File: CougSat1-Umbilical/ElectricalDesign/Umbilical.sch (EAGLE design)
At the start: 48 parts, among them J1 USB, J2 Umbilical, J3 5V input, Q1 CSD16406Q3, Q2 CSD16406Q3, U1 FT230XQ, U2 BQ24650

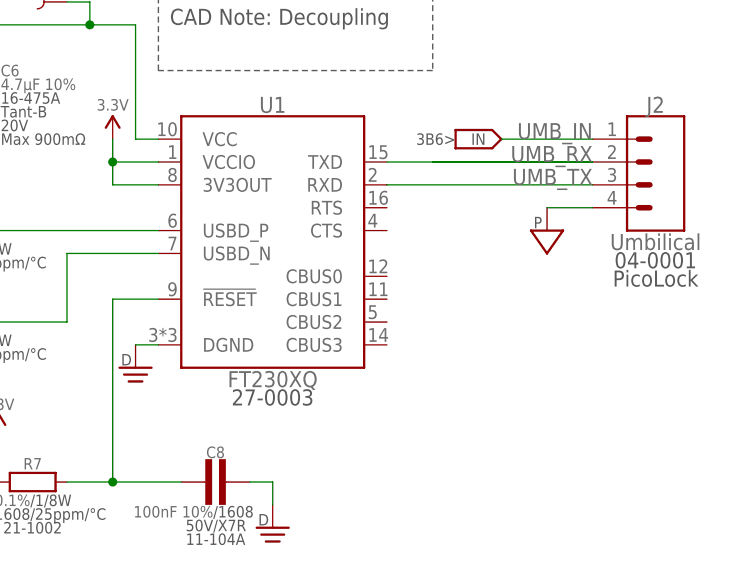
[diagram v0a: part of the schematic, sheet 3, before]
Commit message: Exported PDF
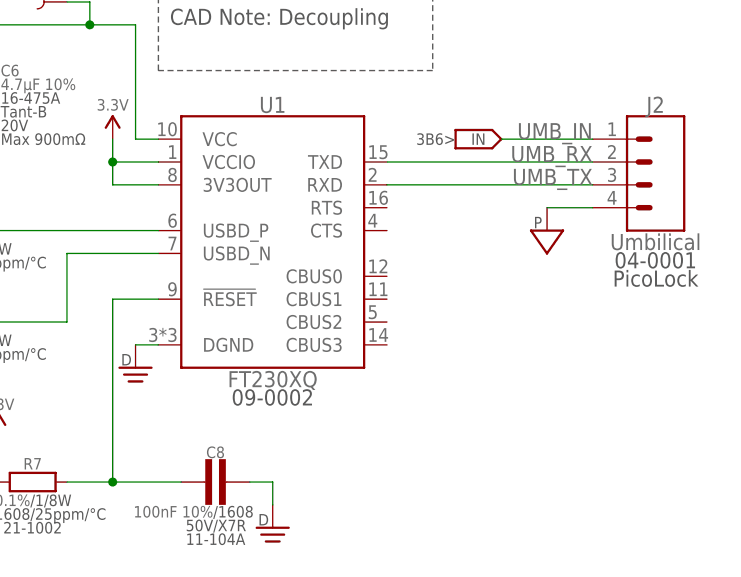
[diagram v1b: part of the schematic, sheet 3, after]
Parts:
- U1: device CougsInSpace-IC-Conversion:FT230X-QFN16 -> CougsInSpace-IC-Comms:FT230X-QFN16
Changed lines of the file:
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@@
 <grid distance="0.1" unitdist="inch" unit="inch" style="lines" multiple="1" display="no" altdistance="0.01" altunitdist="inch" altunit="inch"/>
 <layers>
-<layer number="1" name="Top" color="4" fill="1" visible="yes" active="no"/>
-<layer number="2" name="Route2" color="16" fill="1" visible="yes" active="no"/>
-<layer number="3" name="Route3" color="17" fill="1" visible="yes" active="no"/>
-<layer number="4" name="Route4" color="18" fill="1" visible="yes" active="no"/>
-<layer number="5" name="Route5" color="19" fill="1" visible="yes" active="no"/>
-<layer number="6" name="Route6" color="25" fill="1" visible="yes" active="no"/>
-<layer number="7" name="Route7" color="26" fill="1" visible="yes" active="no"/>
-<layer number="8" name="Route8" color="27" fill="1" visible="yes" active="no"/>
-<layer number="9" name="Route9" color="28" fill="1" visible="yes" active="no"/>
-<layer number="10" name="Route10" color="29" fill="1" visible="yes" active="no"/>
-<layer number="11" name="Route11" color="30" fill="1" visible="yes" active="no"/>
-<layer number="12" name="Route12" color="20" fill="1" visible="yes" active="no"/>
-<layer number="13" name="Route13" color="21" fill="1" visible="yes" active="no"/>
-<layer number="14" name="Route14" color="22" fill="1" visible="yes" active="no"/>
-<layer number="15" name="Route15" color="23" fill="1" visible="yes" active="no"/>
-<layer number="16" name="Bottom" color="1" fill="1" visible="yes" active="no"/>
-<layer number="17" name="Pads" color="2" fill="1" visible="yes" active="no"/>
-<layer number="18" name="Vias" color="2" fill="1" visible="yes" active="no"/>
-<layer number="19" name="Unrouted" color="6" fill="1" visible="yes" active="no"/>
-<layer number="20" name="Dimension" color="24" fill="1" visible="yes" active="no"/>
-<layer number="21" name="tPlace" color="7" fill="1" visible="yes" active="no"/>
-<layer number="22" name="bPlace" color="7" fill="1" visible="yes" active="no"/>
-<layer number="23" name="tOrigins" color="15" fill="1" visible="yes" active="no"/>
-<layer number="24" name="bOrigins" color="15" fill="1" visible="yes" active="no"/>
-<layer number="25" name="tNames" color="7" fill="1" visible="yes" active="no"/>
-<layer number="26" name="bNames" color="7" fill="1" visible="yes" active="no"/>
-<layer number="27" name="tValues" color="7" fill="1" visible="yes" active="no"/>
-<layer number="28" name="bValues" color="7" fill="1" visible="yes" active="no"/>
+<layer number="1" name="Top" color="4" fill="1" visible="no" active="no"/>
+<layer number="2" name="Route2" color="16" fill="1" visible="no" active="no"/>
+<layer number="3" name="Route3" color="17" fill="1" visible="no" active="no"/>
+<layer number="4" name="Route4" color="18" fill="1" visible="no" active="no"/>
+<layer number="5" name="Route5" color="19" fill="1" visible="no" active="no"/>
+<layer number="6" name="Route6" color="25" fill="1" visible="no" active="no"/>
+<layer number="7" name="Route7" color="26" fill="1" visible="no" active="no"/>
+<layer number="8" name="Route8" color="27" fill="1" visible="no" active="no"/>
+<layer number="9" name="Route9" color="28" fill="1" visible="no" active="no"/>
+<layer number="10" name="Route10" color="29" fill="1" visible="no" active="no"/>
+<layer number="11" name="Route11" color="30" fill="1" visible="no" active="no"/>
+<layer number="12" name="Route12" color="20" fill="1" visible="no" active="no"/>
+<layer number="13" name="Route13" color="21" fill="1" visible="no" active="no"/>
+<layer number="14" name="Route14" color="22" fill="1" visible="no" active="no"/>
+<layer number="15" name="Route15" color="23" fill="1" visible="no" active="no"/>
+<layer number="16" name="Bottom" color="1" fill="1" visible="no" active="no"/>
+<layer number="17" name="Pads" color="2" fill="1" visible="no" active="no"/>
+<layer number="18" name="Vias" color="2" fill="1" visible="no" active="no"/>
+<layer number="19" name="Unrouted" color="6" fill="1" visible="no" active="no"/>
+<layer number="20" name="Dimension" color="24" fill="1" visible="no" active="no"/>
+<layer number="21" name="tPlace" color="7" fill="1" visible="no" active="no"/>
+<layer number="22" name="bPlace" color="7" fill="1" visible="no" active="no"/>
+<layer number="23" name="tOrigins" color="15" fill="1" visible="no" active="no"/>
+<layer number="24" name="bOrigins" color="15" fill="1" visible="no" active="no"/>
+<layer number="25" name="tNames" color="7" fill="1" visible="no" active="no"/>
+<layer number="26" name="bNames" color="7" fill="1" visible="no" active="no"/>
+<layer number="27" name="tValues" color="7" fill="1" visible="no" active="no"/>
+<layer number="28" name="bValues" color="7" fill="1" visible="no" active="no"/>
 <layer number="29" name="tStop" color="7" fill="3" visible="no" active="no"/>
 <layer number="30" name="bStop" color="7" fill="6" visible="no" active="no"/>
@@
 <layer number="35" name="tGlue" color="7" fill="4" visible="no" active="no"/>
 <layer number="36" name="bGlue" color="7" fill="5" visible="no" active="no"/>
-<layer number="37" name="tTest" color="7" fill="1" visible="yes" active="no"/>
-<layer number="38" name="bTest" color="7" fill="1" visible="yes" active="no"/>
+<layer number="37" name="tTest" color="7" fill="1" visible="no" active="no"/>
+<layer number="38" name="bTest" color="7" fill="1" visible="no" active="no"/>
 <layer number="39" name="tKeepout" color="4" fill="11" visible="no" active="no"/>
 <layer number="40" name="bKeepout" color="1" fill="11" visible="no" active="no"/>
@@
 <layer number="44" name="Drills" color="7" fill="1" visible="no" active="no"/>
 <layer number="45" name="Holes" color="7" fill="1" visible="no" active="no"/>
-<layer number="46" name="Milling" color="3" fill="1" visible="yes" active="no"/>
-<layer number="47" name="Measures" color="7" fill="1" visible="yes" active="no"/>
-<layer number="48" name="Document" color="7" fill="1" visible="yes" active="no"/>
-<layer number="49" name="Reference" color="7" fill="1" visible="yes" active="no"/>
-<layer number="50" name="dxf" color="7" fill="1" visible="yes" active="no"/>
-<layer number="51" name="tDocu" color="7" fill="1" visible="yes" active="no"/>
-<layer number="52" name="bDocu" color="7" fill="1" visible="yes" active="no"/>
-<layer number="53" name="tGND_GNDA" color="7" fill="9" visible="yes" active="no"/>
-<layer number="54" name="bGND_GNDA" color="1" fill="9" visible="yes" active="no"/>
-<layer number="56" name="wert" color="7" fill="1" visible="yes" active="no"/>
-<layer number="57" name="tCAD" color="7" fill="1" visible="yes" active="no"/>
-<layer number="58" name="bCAD" color="9" fill="1" visible="yes" active="no"/>
-<layer number="59" name="tCarbon" color="7" fill="1" visible="yes" active="no"/>
-<layer number="60" name="bCarbon" color="7" fill="1" visible="yes" active="no"/>
+<layer number="46" name="Milling" color="3" fill="1" visible="no" active="no"/>
+<layer number="47" name="Measures" color="7" fill="1" visible="no" active="no"/>
+<layer number="48" name="Document" color="7" fill="1" visible="no" active="no"/>
+<layer number="49" name="Reference" color="7" fill="1" visible="no" active="no"/>
+<layer number="50" name="dxf" color="7" fill="1" visible="no" active="no"/>
+<layer number="51" name="tDocu" color="7" fill="1" visible="no" active="no"/>
+<layer number="52" name="bDocu" color="7" fill="1" visible="no" active="no"/>
+<layer number="53" name="tGND_GNDA" color="7" fill="9" visible="no" active="no"/>
+<layer number="54" name="bGND_GNDA" color="1" fill="9" visible="no" active="no"/>
+<layer number="56" name="wert" color="7" fill="1" visible="no" active="no"/>
+<layer number="57" name="tCAD" color="7" fill="1" visible="no" active="no"/>
+<layer number="58" name="bCAD" color="9" fill="1" visible="no" active="no"/>
+<layer number="59" name="tCarbon" color="7" fill="1" visible="no" active="no"/>
+<layer number="60" name="bCarbon" color="7" fill="1" visible="no" active="no"/>
 <layer number="88" name="SimResults" color="9" fill="1" visible="yes" active="yes"/>
 <layer number="89" name="SimProbes" color="9" fill="1" visible="yes" active="yes"/>
@@
 <layer number="91" name="Nets" color="2" fill="1" visible="yes" active="yes"/>
 <layer number="92" name="Busses" color="1" fill="1" visible="yes" active="yes"/>
-<layer number="93" name="Pins" color="2" fill="1" visible="no" active="yes"/>
+<layer number="93" name="Pins" color="2" fill="1" visible="yes" active="yes"/>
 <layer number="94" name="Symbols" color="4" fill="1" visible="yes" active="yes"/>
 <layer number="95" name="Names" color="7" fill="1" visible="yes" active="yes"/>
@@
 <attribute name="TITLE" value="Serial Transceiver"/>
 </part>
-<part name="U1" library="CougsInSpace-IC-Conversion" deviceset="FT230X" device="-QFN16" value="FT230XQ"/>
+<part name="U1" library="CougsInSpace-IC-Comms" deviceset="FT230X" device="-QFN16" value="FT230XQ"/>
 <part name="J1" library="CougsInSpace-Connectors" deviceset="USB" device="-B-FEMALE" value="USB"/>
 <part name="J2" library="CougsInSpace-Connectors" deviceset="1X04" device="-PICOLOCK" value="Umbilical"/>
@@
 <segment>
 <pinref part="J2" gate="G$1" pin="2"/>
-<wire x1="185.42" y1="127" x2="167.64" y2="127" width="0.1524" layer="91"/>
 <pinref part="U1" gate="G$1" pin="TXD"/>
 <wire x1="185.42" y1="127" x2="162.56" y2="127" width="0.1524" layer="91"/>
@@
 </sheet>
 </sheets>
+<errors>
+</errors>
 </schematic>
 </drawing>
